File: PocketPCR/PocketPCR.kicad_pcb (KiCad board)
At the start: 2 copper layers, 91.7 x 76.2 mm, 29 parts, among them J1 LID, J2 BLOCK, J3 FAN, J4 PELTIER, J5 USB_PD, Q1 IRF9540N, Q2 IRF540N, Q3 IRF9540N, Q4 IRF540N, Q5 DMG2301L, U1 NTR3C21NZT1G, U2 RaspberryPi_Pico, U3 L7805, U5 L293D

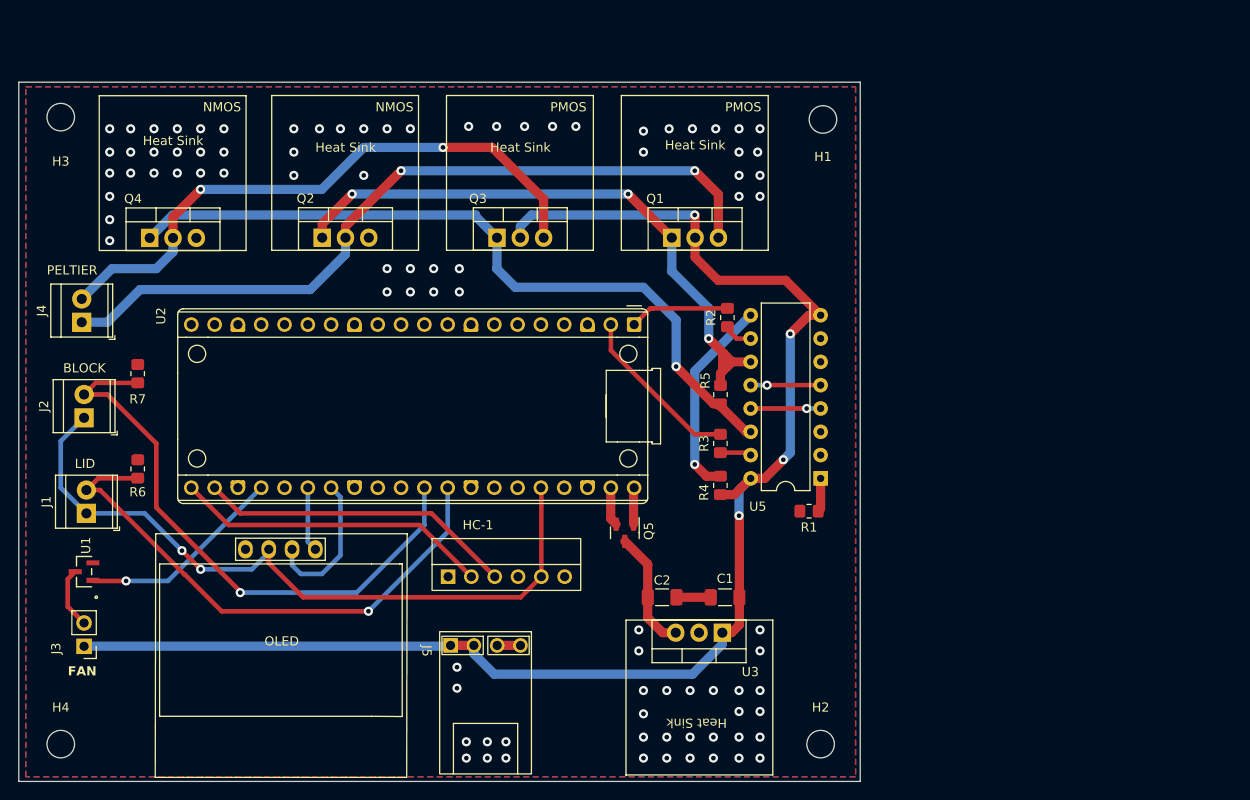
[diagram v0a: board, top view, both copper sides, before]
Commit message: PCB Version 4
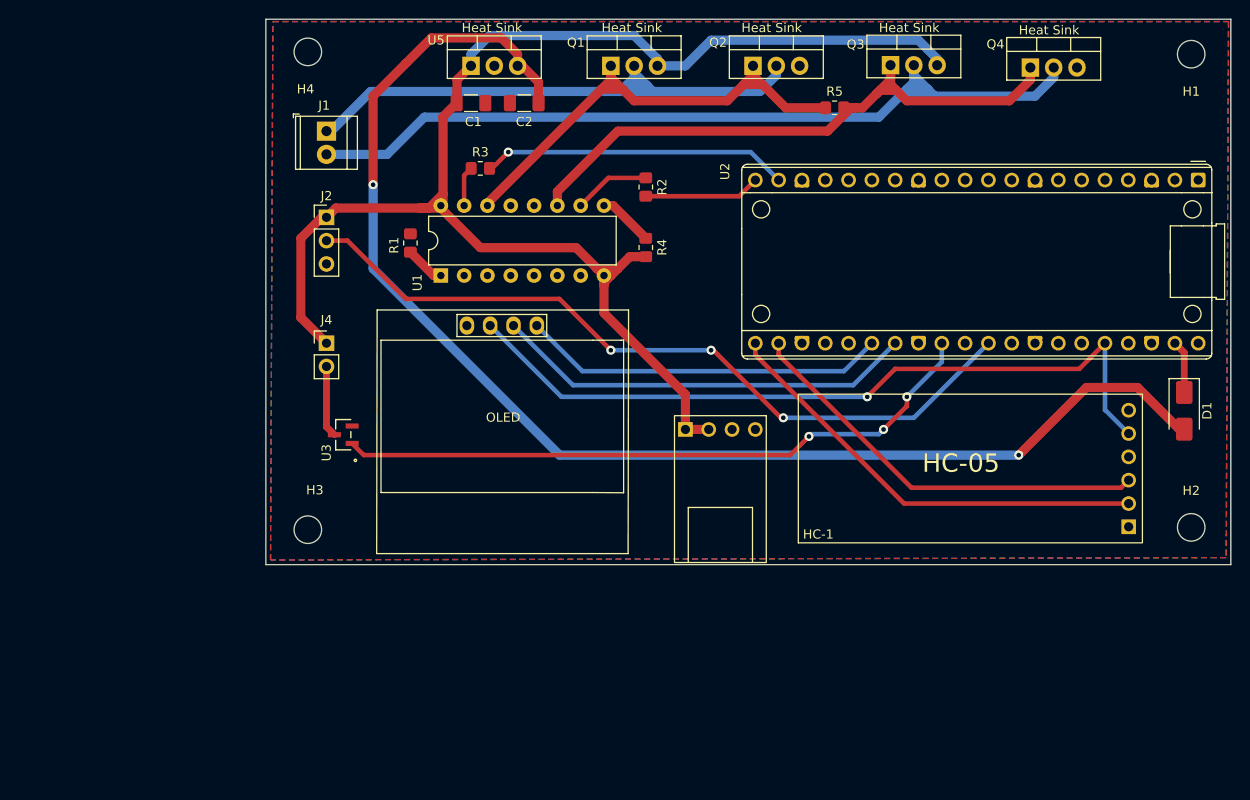
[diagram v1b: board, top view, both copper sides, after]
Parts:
- removed the J4 at (88.6, 77.0)
- removed Q5: DMG2301L, Package_TO_SOT_SMD:SOT-23
- removed R6, R7: 10k, Resistor_SMD:R_0805_2012Metric_Pad1.20x1.40mm_HandSolder
- removed the U1 at (88.9, 104.1)
- added D1: B160-E3, Diode_SMD:D_SMA, F.Cu at (208.8, 86.6)
- added U3: NTR3C21NZT1G, footprints:SOT-23_ONS, F.Cu at (117.1, 89.2)
- HC-1: footprint Custom_footprints:HC05-Vertical -> Custom_footprints:HC-05
- J1: value LID -> PELTIER
- J2: footprint TerminalBlock_TE-Connectivity:TerminalBlock_TE_282834-2_1x02_P2.54mm_Horizontal -> Connector_PinHeader_2.54mm:PinHeader_1x03_P2.54mm_Vertical
- moved Q4 97.8 mm to (192.0, 49.2)
- moved H4 80.1 mm to (113.3, 47.5)
- moved U5 67.6 mm to (131.1, 49.0), turned to 0 degrees
- moved U2 63.5 mm to (186.2, 70.4)
- moved C1 60.5 mm to (131.1, 53.1), turned to 0 degrees
- moved C2 55.9 mm to (136.9, 53.1), turned to 180 degrees
- moved H3 52.4 mm to (113.3, 99.6)
- moved R1 52.4 mm to (124.5, 68.3), turned to -90 degrees
- moved Q2 50.5 mm to (161.8, 49.0)
- moved J1 49.2 mm to (115.3, 56.1), turned to -90 degrees
- moved U1 46.9 mm to (127.8, 71.9), turned to 90 degrees
- moved Q3 46.8 mm to (176.8, 49.0)
- moved H2 46.8 mm to (209.6, 99.3)
- moved J4 42.3 mm to (115.3, 79.2), turned to 0 degrees
- moved H1 40.8 mm to (209.6, 47.8)
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- renumbered J5 to J3, J3 to J4, U5 to U1, U3 to U5
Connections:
- net /BLOCK renamed /BLOCK_ADC
- J1 pad 1: /3.3V -> /HBRG_OUT1
- J1 pad 2: /LID -> /HBRG_OUT2
- J2 pad 1: /3.3V -> V_USB
- Q1 pad 2: V_USB -> /HBRG_OUT1
- Q1 pad 3: /HBRG_OUT1 -> V_USB
- Q3 pad 2: V_USB -> /HBRG_OUT2
- Q3 pad 3: /HBRG_OUT2 -> V_USB
- R2 pad 1: /MD_IN1 -> /MD_IN2
- R3 pad 1: /MD_IN2 -> /MD_IN1
- R5 pad 1: /HBRG_IN2 -> /HBRG_IN1
- R5 pad 2: /HBRG_IN1 -> /HBRG_IN2
- U1 pad 11: /HBRG_IN1 -> /HBRG_IN2
- U1 pad 14: /HBRG_IN2 -> /HBRG_IN1
- U2 pad 1: /MD_IN1 -> unconnected-(U2-GPIO0-Pad1)
- U2 pad 19: unconnected-(U2-GPIO14-Pad19) -> /MD_IN1
- U2 pad 2: /MD_IN2 -> unconnected-(U2-GPIO1-Pad2)
- U2 pad 20: unconnected-(U2-GPIO15-Pad20) -> /MD_IN2
- U2 pad 24: /FAN -> unconnected-(U2-GPIO18-Pad24)
- U2 pad 29: unconnected-(U2-GPIO22-Pad29) -> /FAN
- U2 pad 32: /LID -> unconnected-(U2-GPIO27_ADC1-Pad32)
- U2 pad 40: Net-(Q5-G) -> unconnected-(U2-VBUS-Pad40)
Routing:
- net V_REG: track 13.1 -> 146.5 mm, vias 0 -> 2
- net /LID: track 59.1 -> 0.00 mm, vias 1 -> 0
- net /FAN: track 23.1 -> 71.6 mm, vias 1 -> 3
- net /SDA: track 7.05 -> 39.8 mm
- net /SCL: track 16.0 -> 46.2 mm
- net /HBRG_OUT2: track 65.9 -> 94.8 mm, vias 2 -> 0
- net /MD_IN1: track 10.9 -> 33.5 mm, vias 0 -> 1
- net GND: track 21.5 -> 0.00 mm, vias 2 -> 0
- net /HBRG_OUT1: track 83.8 -> 62.4 mm, vias 2 -> 0
- net /BLOCK_ADC: track 63.7 -> 83.5 mm, vias 1 -> 3
- net Net-(U1-EN3,4): track 22.1 -> 6.03 mm, vias 1 -> 0
- net /BLUE_RX: track 34.5 -> 48.7 mm
- net /HBRG_IN2: track 81.6 -> 69.2 mm, vias 1 -> 0
- net /HBRG_IN1: track 66.5 -> 54.6 mm, vias 3 -> 0
- net /BLUE_TX: track 34.5 -> 45.7 mm
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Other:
- board size 91.7 x 76.2 mm -> 105.2 x 59.4 mm
- board text added: "H4"
- board text added: "MH4"
- board text added: "POCKET PCR TUE-16"
- board text removed: "BLOCK"
- board text removed: "FAN"
- board text removed: "LID"
- board text removed: "NMOS"
- board text removed: "PELTIER"
- board text removed: "PMOS"
